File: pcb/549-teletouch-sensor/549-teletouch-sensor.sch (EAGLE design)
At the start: 87 parts, among them J1 RASPBERRYPI-40-PIN-GPIO_PTH, J2 RASPBERRYPI-40-PIN-GPIO_PTH

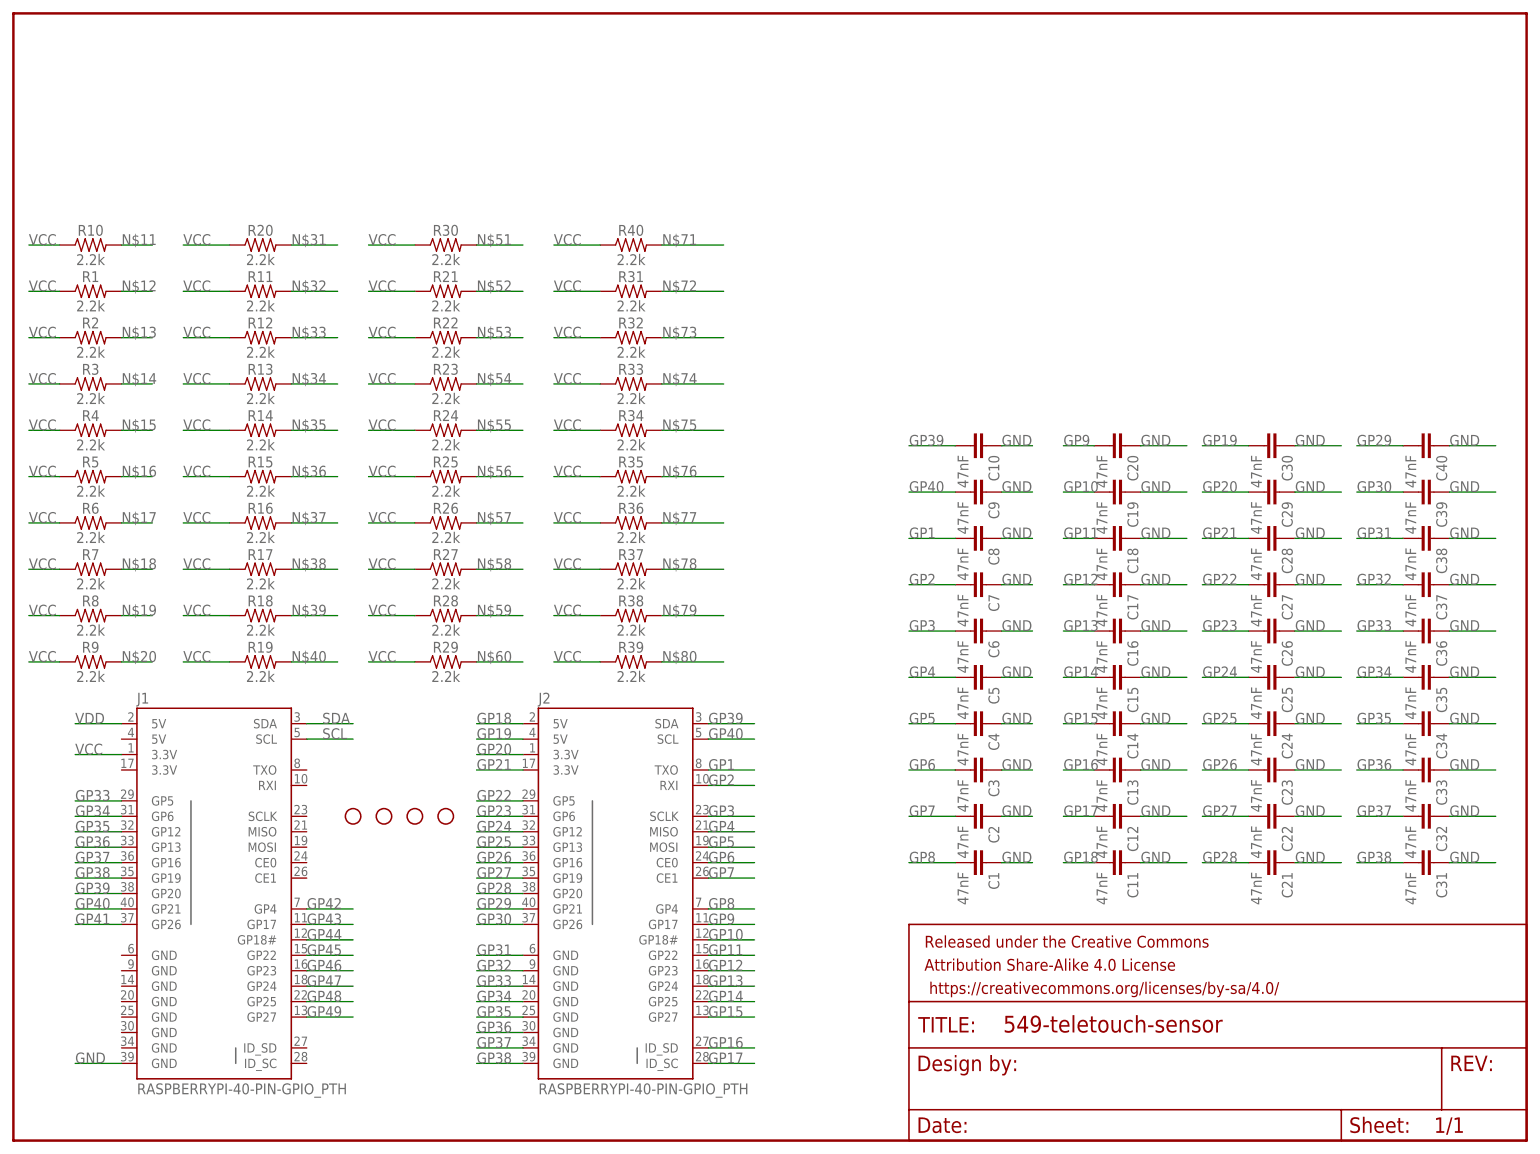
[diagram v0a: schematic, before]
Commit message: updated sensor pcb
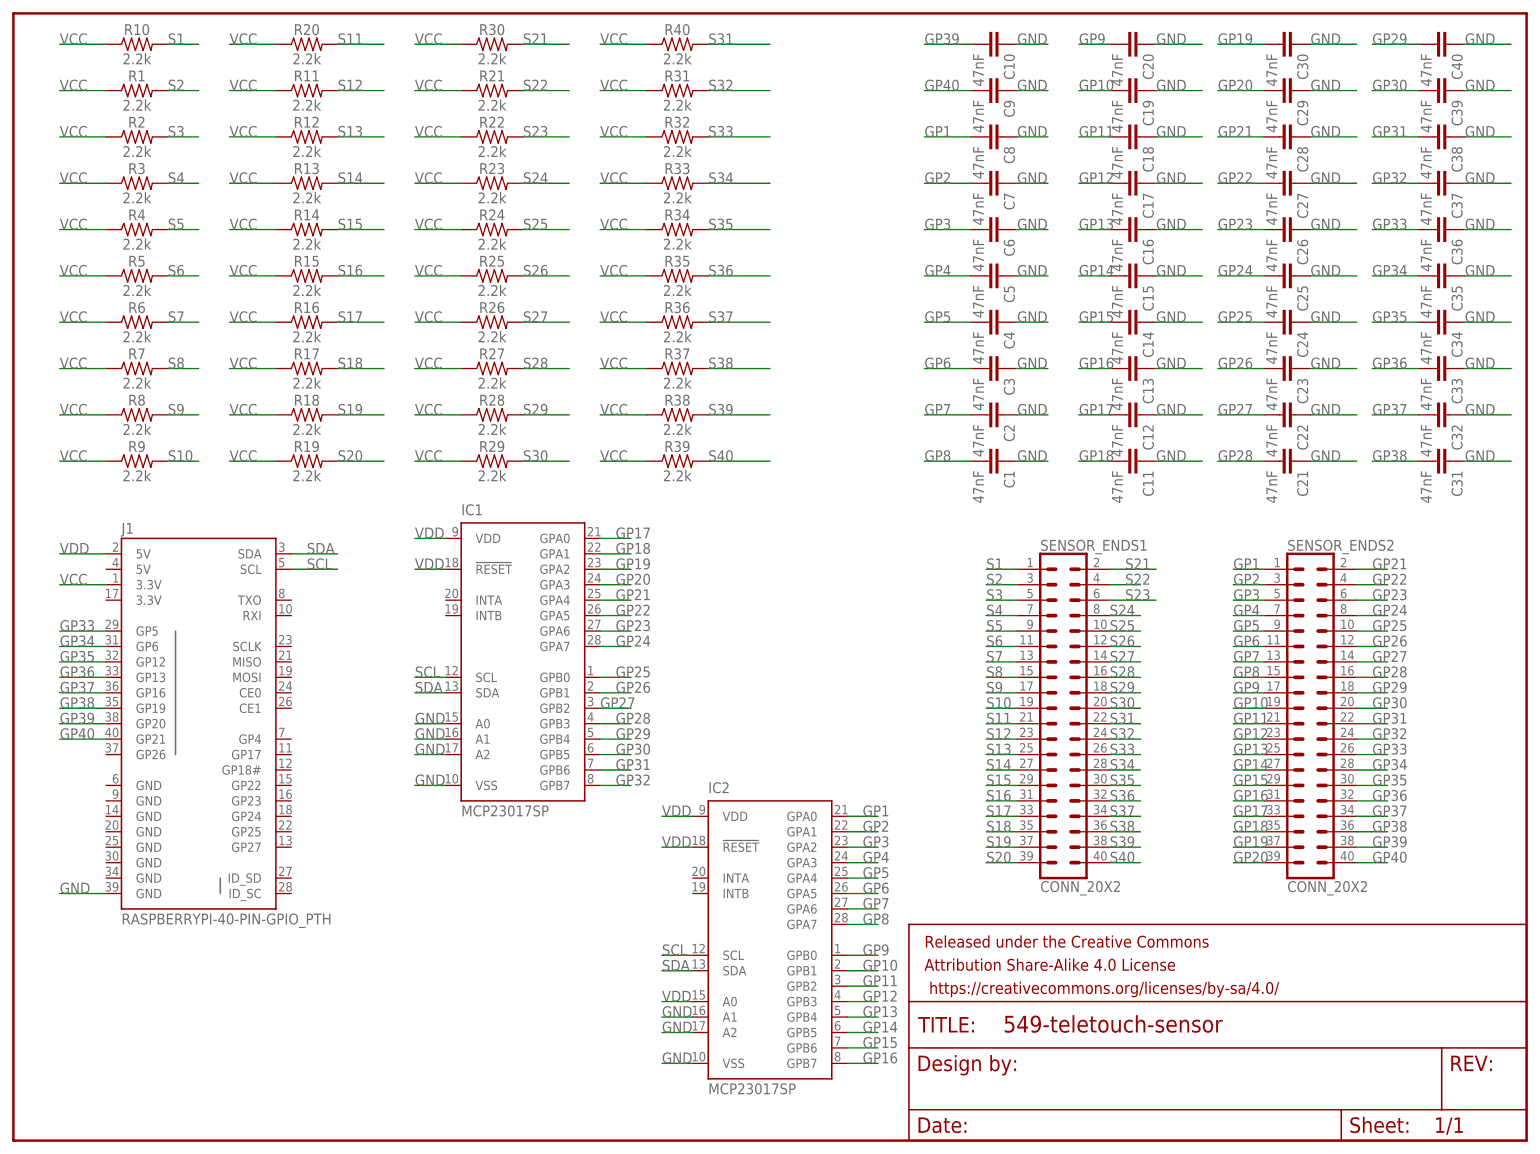
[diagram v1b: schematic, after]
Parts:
- removed H1, H2, H3, H4: STAND-OFF, SparkFun-Hardware:STAND-OFF
- removed J2: RASPBERRYPI-40-PIN-GPIO_PTH, SparkFun-Connectors:RASPBERRYPI-40-PIN-GPIO_PTH
- added IC1, IC2: MCP23017SP, adafruit:MCP23017SP
- added SENSOR_ENDS1, SENSOR_ENDS2: CONN_20X2, SparkFun-Connectors:CONN_20X2
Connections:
- removed net GP41: J1.GP26
- removed net GP42: J1.GP4
- removed net GP43: J1.GP17
- removed net GP44: J1.GP18#
- removed net GP45: J1.GP22
- removed net GP46: J1.GP23
- removed net GP47: J1.GP24
- removed net GP48: J1.GP25
- removed net GP49: J1.GP27
- removed net N$11: R10.2
- removed net N$12: R1.2
- removed net N$13: R2.2
- removed net N$14: R3.2
- removed net N$15: R4.2
- removed net N$16: R5.2
- removed net N$17: R6.2
- removed net N$18: R7.2
- removed net N$19: R8.2
- removed net N$20: R9.2
- removed net N$31: R20.2
- removed net N$32: R11.2
- removed net N$33: R12.2
- removed net N$34: R13.2
- removed net N$35: R14.2
- removed net N$36: R15.2
- removed net N$37: R16.2
- removed net N$38: R17.2
- removed net N$39: R18.2
- removed net N$40: R19.2
- removed net N$51: R30.2
- removed net N$52: R21.2
- removed net N$53: R22.2
- removed net N$54: R23.2
- removed net N$55: R24.2
- removed net N$56: R25.2
- removed net N$57: R26.2
- removed net N$58: R27.2
- removed net N$59: R28.2
- removed net N$60: R29.2
- removed net N$71: R40.2
- removed net N$72: R31.2
- removed net N$73: R32.2
- removed net N$74: R33.2
- removed net N$75: R34.2
- removed net N$76: R35.2
- removed net N$77: R36.2
- removed net N$78: R37.2
- removed net N$79: R38.2
- removed net N$80: R39.2
- new net S1: R10.2, SENSOR_ENDS1.1
- new net S10: R9.2, SENSOR_ENDS1.19
- new net S11: R20.2, SENSOR_ENDS1.21
- new net S12: R11.2, SENSOR_ENDS1.23
- new net S13: R12.2, SENSOR_ENDS1.25
- new net S14: R13.2, SENSOR_ENDS1.27
- new net S15: R14.2, SENSOR_ENDS1.29
- new net S16: R15.2, SENSOR_ENDS1.31
- new net S17: R16.2, SENSOR_ENDS1.33
- new net S18: R17.2, SENSOR_ENDS1.35
- new net S19: R18.2, SENSOR_ENDS1.37
- new net S2: R1.2, SENSOR_ENDS1.3
- new net S20: R19.2, SENSOR_ENDS1.39
- new net S21: R30.2, SENSOR_ENDS1.2
- new net S22: R21.2, SENSOR_ENDS1.4
- new net S23: R22.2, SENSOR_ENDS1.6
- new net S24: R23.2, SENSOR_ENDS1.8
- new net S25: R24.2, SENSOR_ENDS1.10
- new net S26: R25.2, SENSOR_ENDS1.12
- new net S27: R26.2, SENSOR_ENDS1.14
- new net S28: R27.2, SENSOR_ENDS1.16
- new net S29: R28.2, SENSOR_ENDS1.18
- new net S3: R2.2, SENSOR_ENDS1.5
- new net S30: R29.2, SENSOR_ENDS1.20
- new net S31: R40.2, SENSOR_ENDS1.22
- new net S32: R31.2, SENSOR_ENDS1.24
- new net S33: R32.2, SENSOR_ENDS1.26
- new net S34: R33.2, SENSOR_ENDS1.28
- new net S35: R34.2, SENSOR_ENDS1.30
- new net S36: R35.2, SENSOR_ENDS1.32
- new net S37: R36.2, SENSOR_ENDS1.34
- new net S38: R37.2, SENSOR_ENDS1.36
- new net S39: R38.2, SENSOR_ENDS1.38
- new net S4: R3.2, SENSOR_ENDS1.7
- new net S40: R39.2, SENSOR_ENDS1.40
- new net S5: R4.2, SENSOR_ENDS1.9
- new net S6: R5.2, SENSOR_ENDS1.11
- new net S7: R6.2, SENSOR_ENDS1.13
- new net S8: R7.2, SENSOR_ENDS1.15
- new net S9: R8.2, SENSOR_ENDS1.17
- net GND: now also IC1.A0, IC1.A1, IC1.A2, IC1.VSS, IC2.A1, IC2.A2, IC2.VSS
- net GP1: now also IC2.GPA0, SENSOR_ENDS2.1; no longer J2.TXO
- net GP10: now also IC2.GPB1, SENSOR_ENDS2.19; no longer J2.GP18#
- net GP11: now also IC2.GPB2, SENSOR_ENDS2.21; no longer J2.GP22
- net GP12: now also IC2.GPB3, SENSOR_ENDS2.23; no longer J2.GP23
- net GP13: now also IC2.GPB4, SENSOR_ENDS2.25; no longer J2.GP24
- net GP14: now also IC2.GPB5, SENSOR_ENDS2.27; no longer J2.GP25
- net GP15: now also IC2.GPB6, SENSOR_ENDS2.29; no longer J2.GP27
- net GP16: now also IC2.GPB7, SENSOR_ENDS2.31; no longer J2.ID_SD
- net GP17: now also IC1.GPA0, SENSOR_ENDS2.33; no longer J2.ID_SC
- net GP18: now also IC1.GPA1, SENSOR_ENDS2.35; no longer J2.5V@2
- net GP19: now also IC1.GPA2, SENSOR_ENDS2.37; no longer J2.5V@4
- net GP2: now also IC2.GPA1, SENSOR_ENDS2.3; no longer J2.RXI
- net GP20: now also IC1.GPA3, SENSOR_ENDS2.39; no longer J2.3.3V@1
- net GP21: now also IC1.GPA4, SENSOR_ENDS2.2; no longer J2.3.3V@17
- net GP22: now also IC1.GPA5, SENSOR_ENDS2.4; no longer J2.GP5
- net GP23: now also IC1.GPA6, SENSOR_ENDS2.6; no longer J2.GP6
- net GP24: now also IC1.GPA7, SENSOR_ENDS2.8; no longer J2.GP12
- net GP25: now also IC1.GPB0, SENSOR_ENDS2.10; no longer J2.GP13
- net GP26: now also IC1.GPB1, SENSOR_ENDS2.12; no longer J2.GP16
- net GP27: now also IC1.GPB2, SENSOR_ENDS2.14; no longer J2.GP19
- net GP28: now also IC1.GPB3, SENSOR_ENDS2.16; no longer J2.GP20
- net GP29: now also IC1.GPB4, SENSOR_ENDS2.18; no longer J2.GP21
- net GP3: now also IC2.GPA2, SENSOR_ENDS2.5; no longer J2.SCLK
- net GP30: now also IC1.GPB5, SENSOR_ENDS2.20; no longer J2.GP26
- net GP31: now also IC1.GPB6, SENSOR_ENDS2.22; no longer J2.GND@6
- net GP32: now also IC1.GPB7, SENSOR_ENDS2.24; no longer J2.GND@9
- net GP33: now also SENSOR_ENDS2.26; no longer J2.GND@14
- net GP34: now also SENSOR_ENDS2.28; no longer J2.GND@20
- net GP35: now also SENSOR_ENDS2.30; no longer J2.GND@25
- net GP36: now also SENSOR_ENDS2.32; no longer J2.GND@30
- net GP37: now also SENSOR_ENDS2.34; no longer J2.GND@34
- net GP38: now also SENSOR_ENDS2.36; no longer J2.GND@39
- net GP39: now also SENSOR_ENDS2.38; no longer J2.SDA
- net GP4: now also IC2.GPA3, SENSOR_ENDS2.7; no longer J2.MISO
- net GP40: now also SENSOR_ENDS2.40; no longer J2.SCL
- net GP5: now also IC2.GPA4, SENSOR_ENDS2.9; no longer J2.MOSI
- net GP6: now also IC2.GPA5, SENSOR_ENDS2.11; no longer J2.CE0
- net GP7: now also IC2.GPA6, SENSOR_ENDS2.13; no longer J2.CE1
- net GP8: now also IC2.GPA7, SENSOR_ENDS2.15; no longer J2.GP4
- net GP9: now also IC2.GPB0, SENSOR_ENDS2.17; no longer J2.GP17
- net SCL: now also IC1.SCL, IC2.SCL
- net SDA: now also IC1.SDA, IC2.SDA
- net VDD: now also IC1.!RESET, IC1.VDD, IC2.!RESET, IC2.A0, IC2.VDD
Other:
- moved on the sheet: C1, C10, C11, C12, C13, C14, C15, C16, C17, C18, C19, C2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
